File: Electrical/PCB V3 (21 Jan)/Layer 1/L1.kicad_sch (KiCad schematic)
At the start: 198 parts, among them J1 Conn_01x02, J3 Conn_01x02, SW1 SW_SPDT, U2 CD74HC4067SM, U3 CD74HC4067SM, U4 XT30UPB-M, U5 113991054

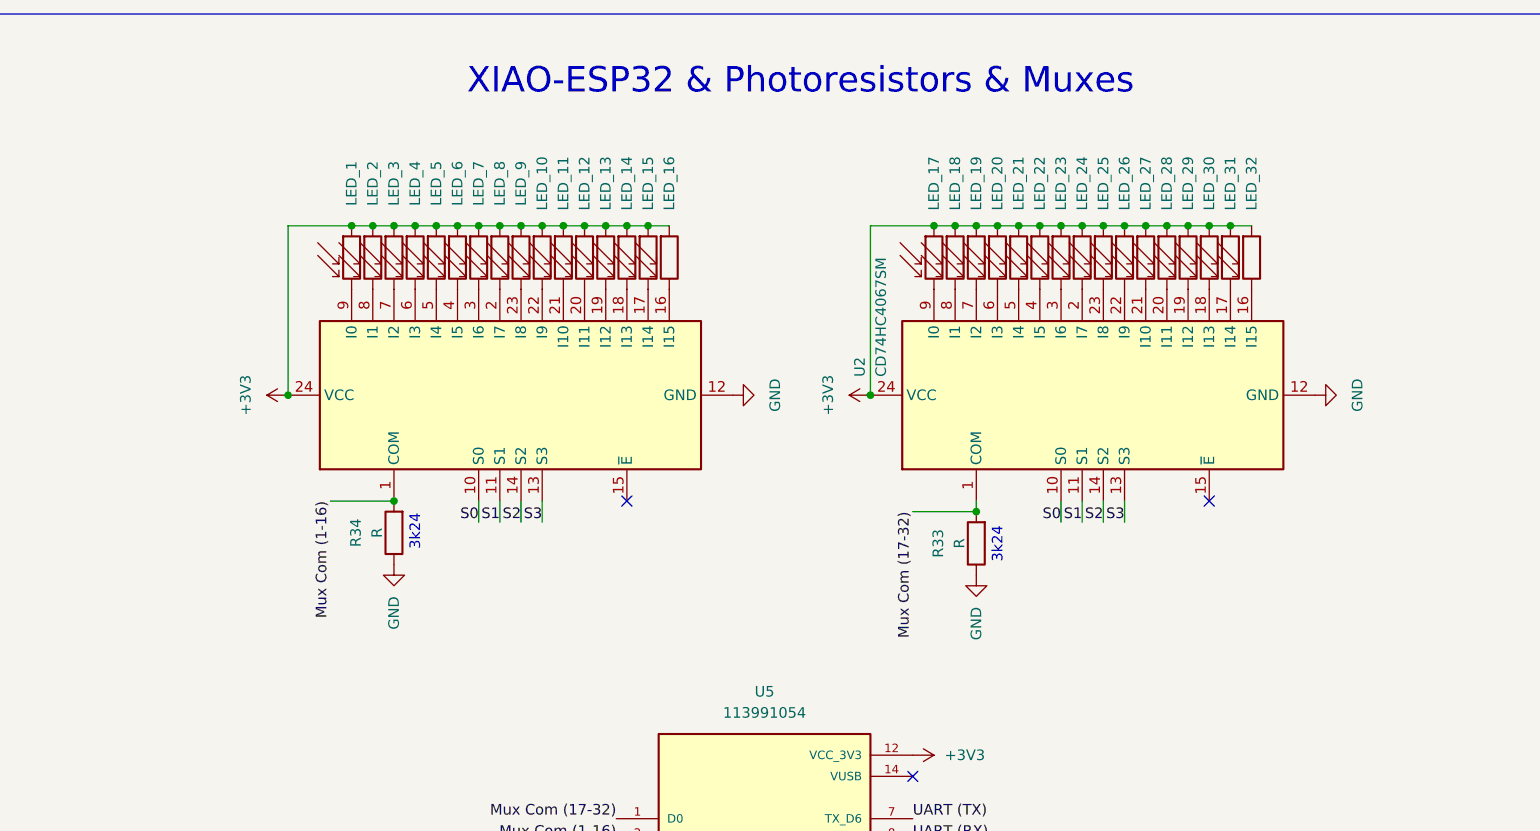
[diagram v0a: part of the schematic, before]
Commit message: finished layer1?
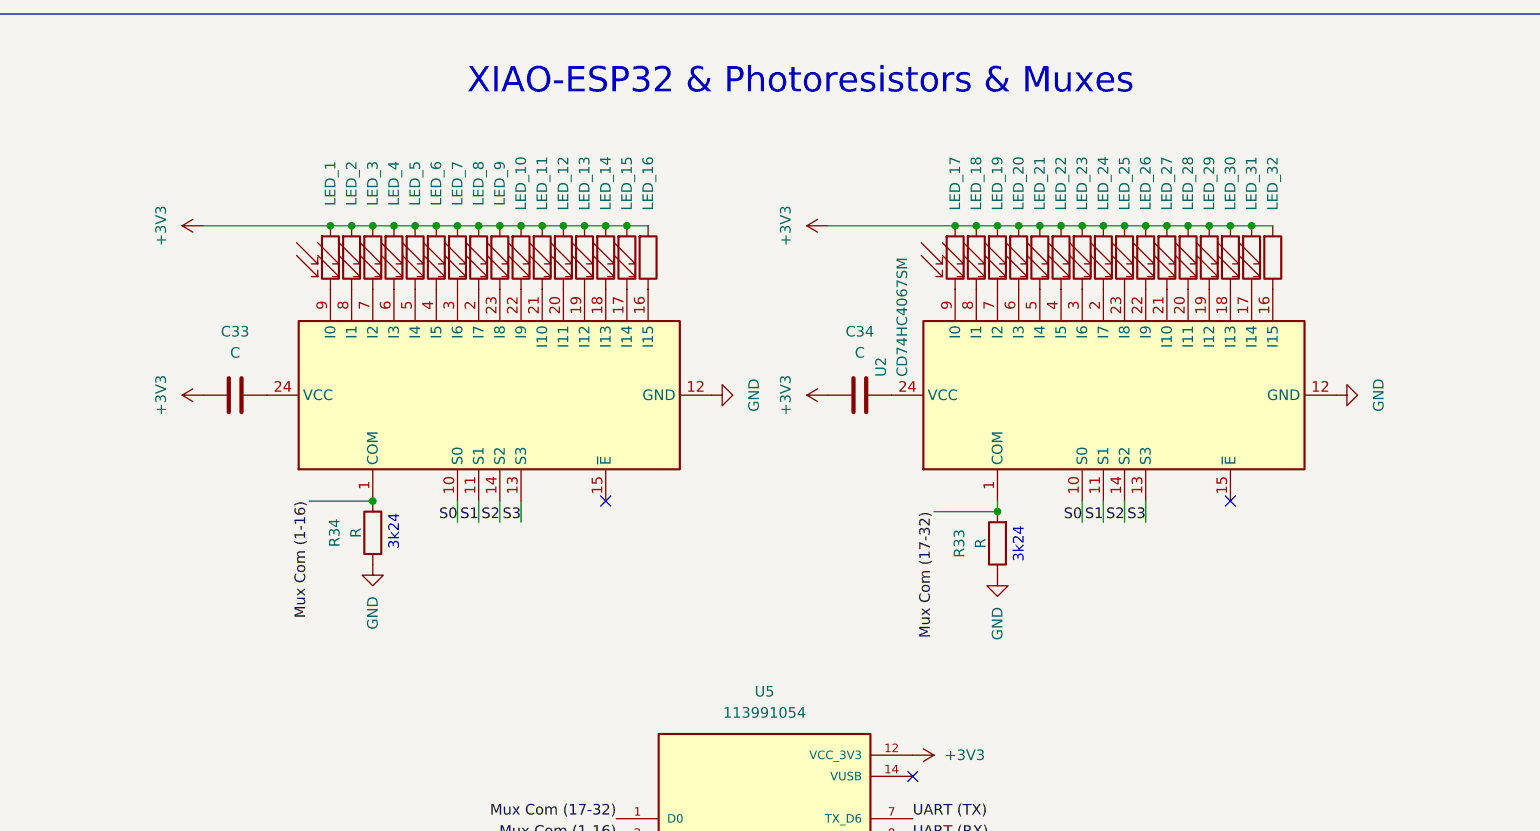
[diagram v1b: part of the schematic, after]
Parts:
- added C33, C34: C, Capacitor_SMD:C_0603_1608Metric, symbol Device:C
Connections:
- net +3V3: now also C33.1, C34.1; no longer U2.24 (VCC), U3.24 (VCC)
- new net: C33.2, U3.24 (VCC)
- new net: C34.2, U2.24 (VCC)
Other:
- moved on the sheet: LED_1, LED_10, LED_11, LED_12, LED_13, LED_14, LED_15, LED_16, LED_17, LED_18, LED_19, LED_2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
